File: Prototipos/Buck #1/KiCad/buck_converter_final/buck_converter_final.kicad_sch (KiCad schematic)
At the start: 25 parts, among them J1 Conn_01x03_Pin, J2 Screw_Terminal_01x02, J3 Screw_Terminal_01x02, Q1 IRF9540NPBF, Q3 NPN

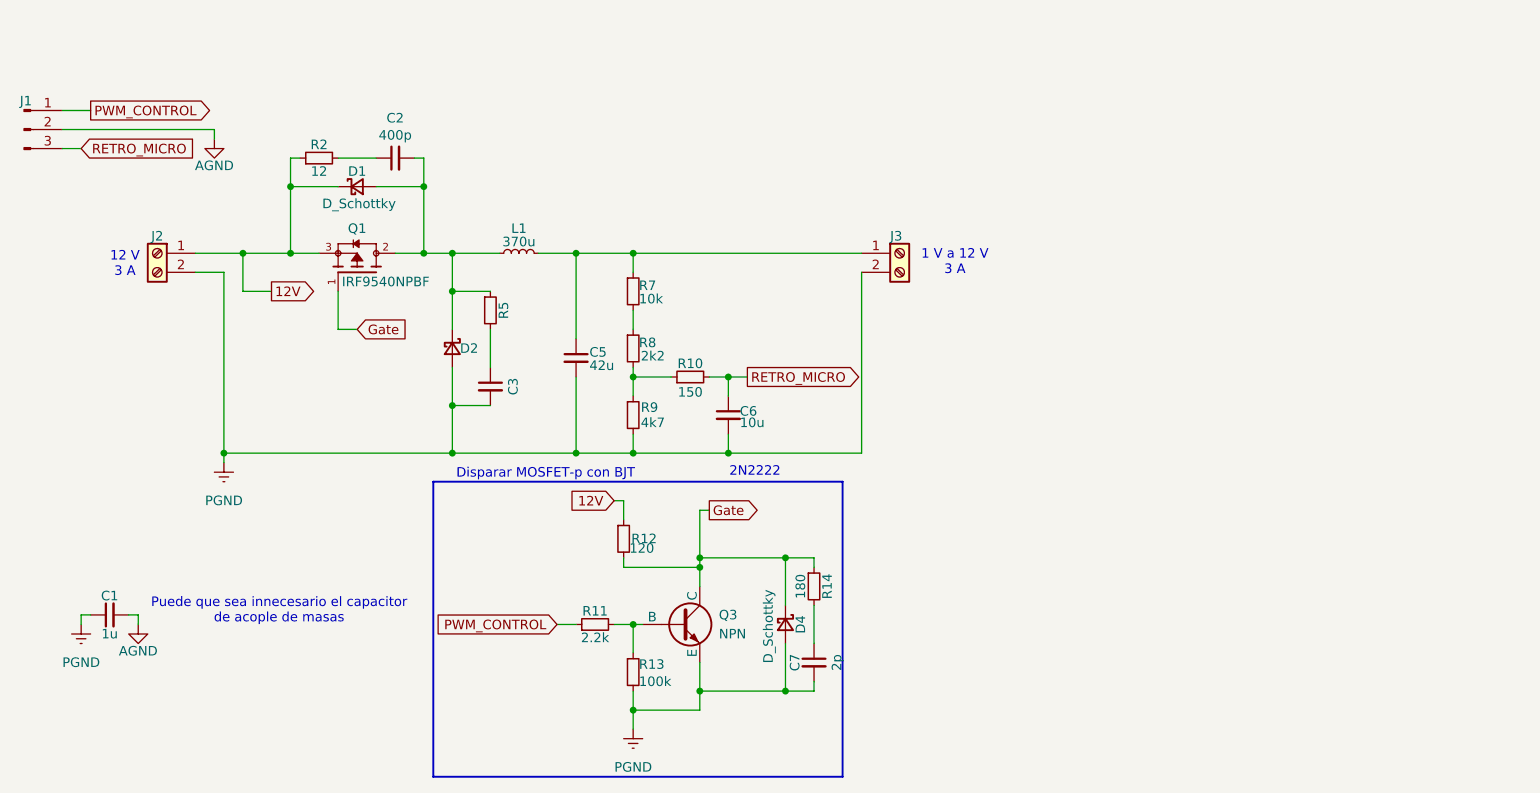
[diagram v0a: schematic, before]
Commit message: Avances PCB convertidor Buck
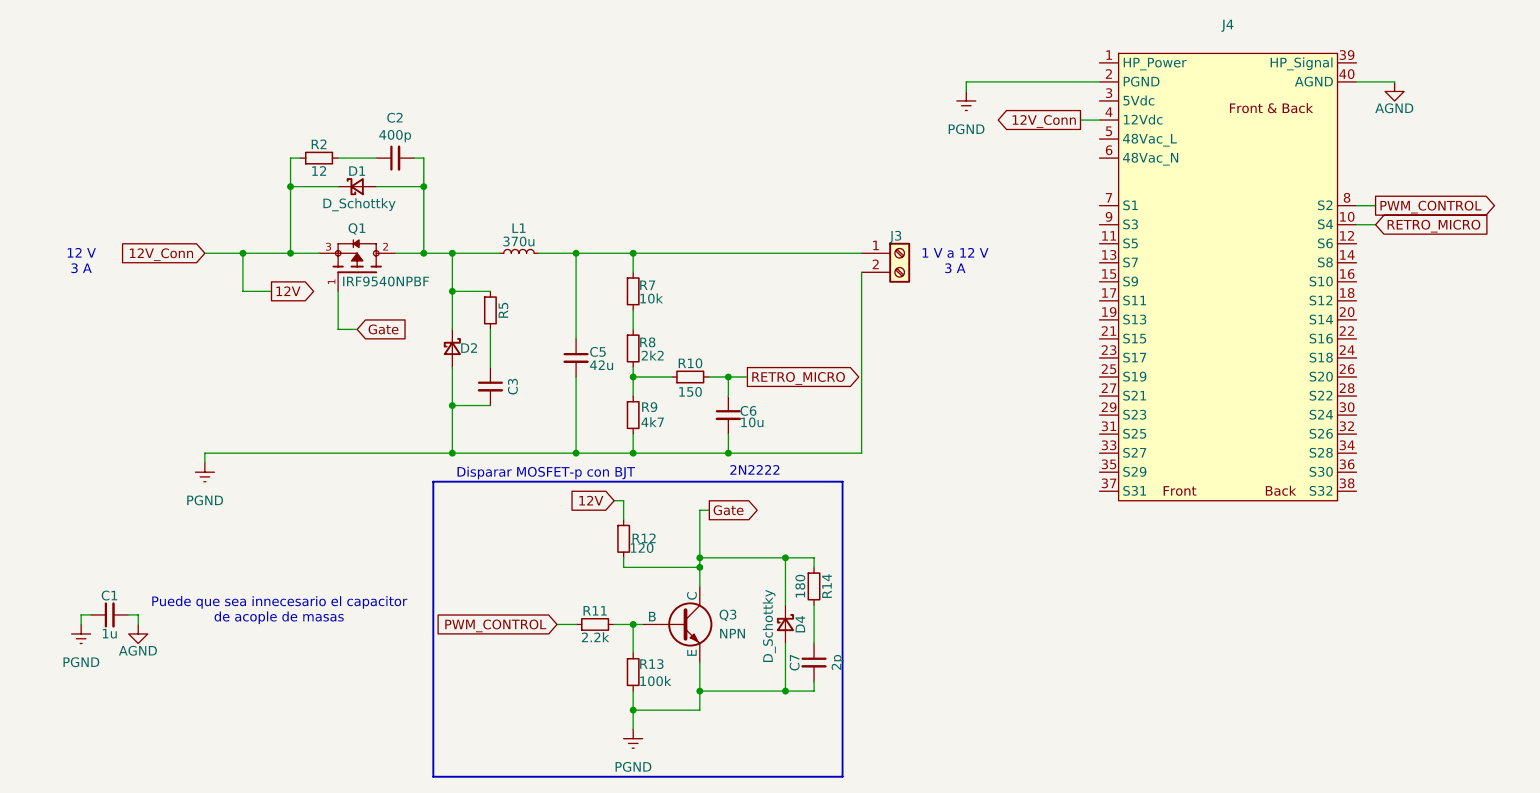
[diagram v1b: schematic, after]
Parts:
- removed J1: Conn_01x03_Pin, Connector_PinHeader_2.54mm:PinHeader_1x03_P2.54mm_Vertical, symbol Connector:Conn_01x03_Pin
- removed J2: Screw_Terminal_01x02, TerminalBlock_Phoenix:TerminalBlock_Phoenix_MKDS-1,5-2-5.08_1x02_P5.08mm_Horizontal, symbol Connector:Screw_Terminal_01x02
- added J4: ~, Proyecto_Final:BUS_PCIE_x4_NSH, symbol Proyecto_Final:PCIE_x4_NSH
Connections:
- net 12V: now also J4.4 (12Vdc)
- net AGND: now also J4.40 (AGND)
- net PGND: now also J4.2 (PGND)
- net PWM_CONTROL: now also J4.8 (S2)
- net RETRO_MICRO: now also J4.10 (S4)

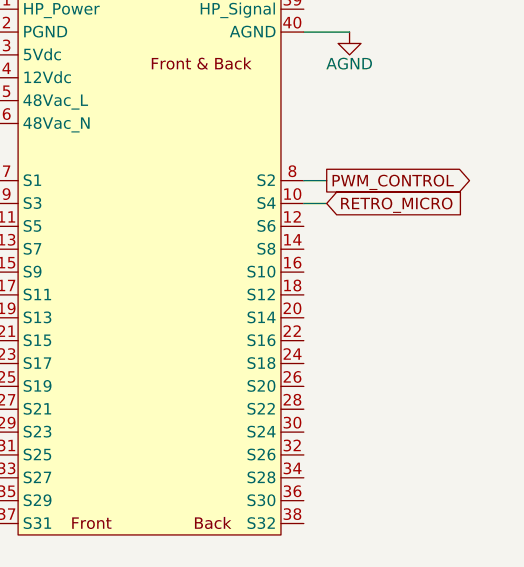
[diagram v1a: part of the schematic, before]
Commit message: Avances en PCB final buck, versión 1.1
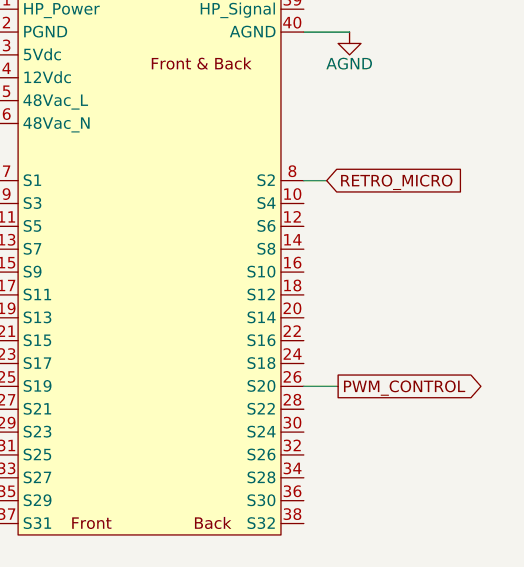
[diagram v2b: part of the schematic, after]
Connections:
- net PWM_CONTROL: now also J4.26 (S20); no longer J4.8 (S2)
- net RETRO_MICRO: now also J4.8 (S2); no longer J4.10 (S4)
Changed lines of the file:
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@@
+	(wire
+		(pts
+			(xy 257.81 71.12) (xy 254 71.12)
+		)
+		(stroke
+			(width 0)
+			(type default)
+		)
+	)
 	(wire
 		(pts
@@
 	(wire
 		(pts
-			(xy 254 50.8) (xy 256.54 50.8)
-		)
-		(stroke
-			(width 0)
-			(type default)
-		)
-	)
-	(wire
-		(pts
 			(xy 149.86 71.12) (xy 149.86 81.28)
 		)
@@
 	(wire
 		(pts
-			(xy 254 48.26) (xy 256.54 48.26)
-		)
-		(stroke
-			(width 0)
-			(type default)
-		)
-	)
-	(wire
-		(pts
 			(xy 167.64 88.9) (xy 166.37 88.9)
+		)
+		(stroke
+			(width 0)
+			(type default)
+		)
+	)
+	(wire
+		(pts
+			(xy 256.54 48.26) (xy 254 48.26)
 		)
 		(stroke
@@
 	(global_label "PWM_CONTROL"
 		(shape output)
-		(at 256.54 48.26 0)
+		(at 257.81 71.12 0)
 		(fields_autoplaced yes)
 		(effects
@@
 		)
 		(property "Intersheetrefs" "${INTERSHEET_REFS}"
-			(at 273.1928 48.26 0)
+			(at 274.4628 71.12 0)
 			(effects
 				(font
@@
 	(global_label "RETRO_MICRO"
 		(shape input)
-		(at 256.54 50.8 0)
+		(at 256.54 48.26 0)
 		(fields_autoplaced yes)
 		(effects
@@
 		)
 		(property "Intersheetrefs" "${INTERSHEET_REFS}"
-			(at 272.4066 50.8 0)
-			(effects
-				(font
+			(at 272.4066 48.26 0)
+			(effects
+				(font
